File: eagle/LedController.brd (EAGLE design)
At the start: 31 parts, among them IC1 MCP601R, Q2 FA-238, Q5 PMV20EN, X2 MKDSN1,5/4-5,08

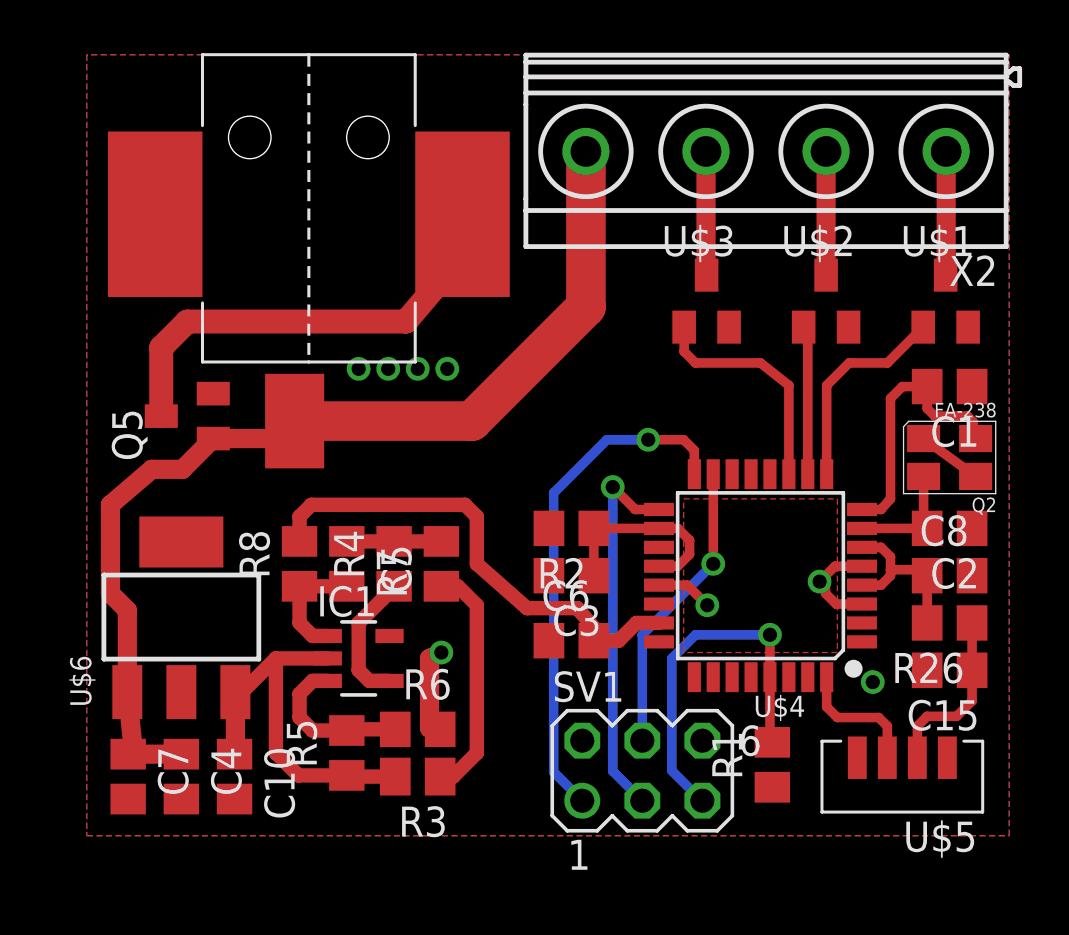
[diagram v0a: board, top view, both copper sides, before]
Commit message: More relayouting, Framed schematic
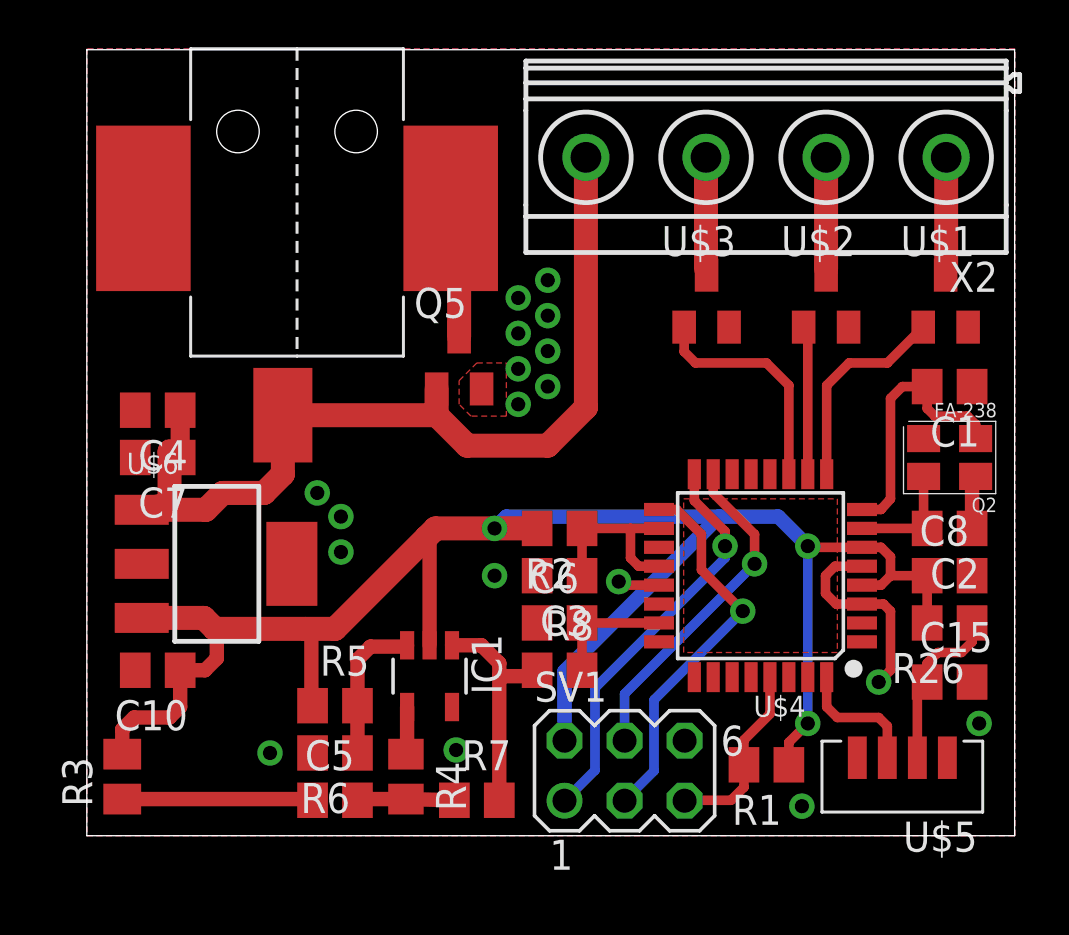
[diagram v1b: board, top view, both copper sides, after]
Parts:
- moved C4 15.5 mm to (3.00, 18.0), turned to 180 degrees
- moved C7 13.6 mm to (3.00, 16.0), turned to 180 degrees
- moved R3 12.5 mm to (1.50, 2.50), turned to 90 degrees
- moved R8 11.9 mm to (20.0, 7.00), turned to 0 degrees
- moved Q5 11.7 mm to (15.8, 20.0), turned to 0 degrees
- moved R7 11.4 mm to (16.5, 1.50), turned to 0 degrees
- moved C5 11.0 mm to (10.5, 1.50), turned to 0 degrees
- moved R4 9.01 mm to (13.5, 2.50), turned to 270 degrees
- moved C10 5.55 mm to (3.00, 7.00), turned to 180 degrees
- moved R6 3.64 mm to (10.5, 3.50), turned to 180 degrees
- moved IC1 3.09 mm to (14.5, 6.75), turned to 180 degrees
- moved U$6 2.70 mm to (5.50, 11.5), turned to 270 degrees
- moved R5 2.06 mm to (10.5, 5.50), turned to 0 degrees
- moved C6 0.90 mm to (20.0, 9.00)
- moved SV1 0.75 mm to (22.8, 2.75)
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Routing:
- net +5V: track 25.5 -> 81.6 mm, vias 0 -> 3
- net ADC: track 20.6 -> 5.46 mm
- net N$8: track 18.9 -> 5.59 mm
- net ISP_RESET: track 15.7 -> 7.86 mm, vias 1 -> 0
- net N$12: track 4.97 -> 10.0 mm
- net +12V: track 45.5 -> 40.8 mm
- net ISP_MISO: track 21.6 -> 17.2 mm
- net N$10: track 5.65 -> 2.00 mm
- net N$1: track 10.0 -> 8.07 mm
- net ISP_MOSI: track 12.5 -> 14.3 mm
- net N$11: track 7.60 -> 6.30 mm
- net GND: track 13.5 -> 12.5 mm, vias 8 -> 18
- net N$9: track 4.00 -> 4.51 mm
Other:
- board outline added: 39.2 x 33.2 mm
